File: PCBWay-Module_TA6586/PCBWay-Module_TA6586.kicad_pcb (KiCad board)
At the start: 2 copper layers, 16.3 x 20.8 mm, 4 parts, among them J1 Conn_01x07_Pin, J2 Conn_01x07_Pin

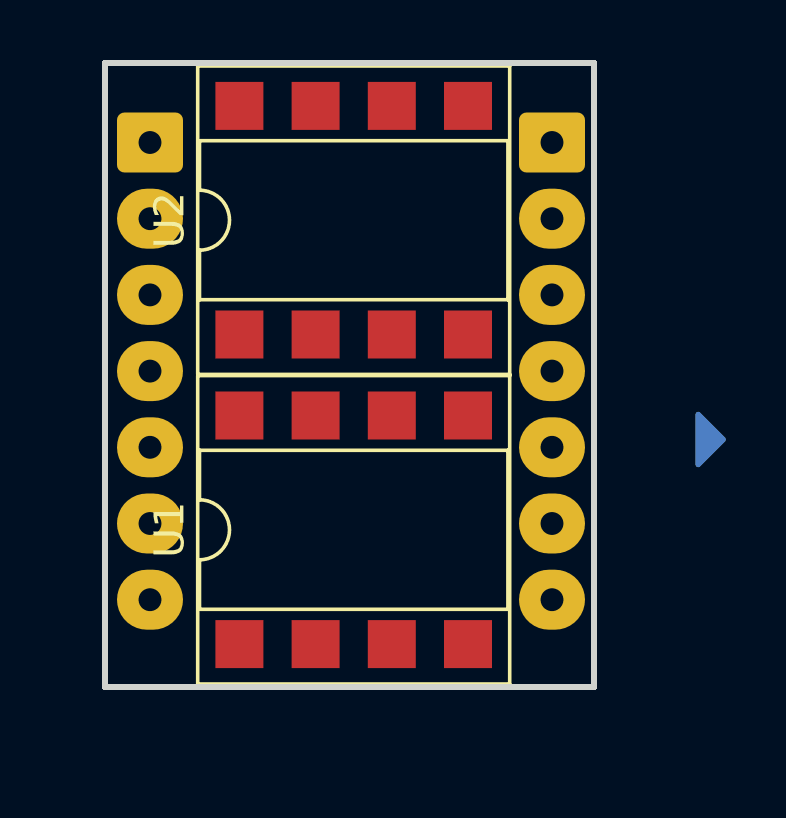
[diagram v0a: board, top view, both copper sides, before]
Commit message: the whole thing
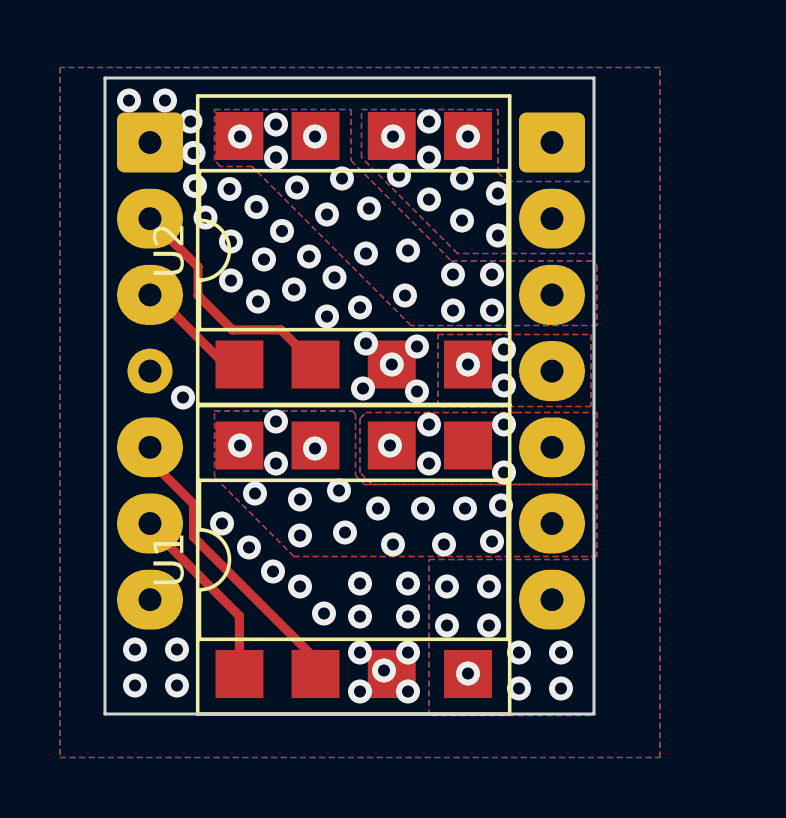
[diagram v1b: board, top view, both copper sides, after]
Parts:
- moved U1 1.00 mm to (146.8, 83.4)
- moved U2 1.00 mm to (146.8, 73.1)
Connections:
- J1 pad 4: unconnected-(J1-Pin_4-Pad4) -> (no net)
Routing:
- net /IN_A2: track 0.00 -> 9.85 mm
- net /IN_B2: track 0.00 -> 8.10 mm
- net /IN_A1: track 0.00 -> 6.25 mm
- net /IN_B1: track 0.00 -> 3.94 mm
- net GND: vias 0 -> 42
- net /VM: vias 0 -> 12
- net /OUT_B2: vias 0 -> 15
- net /OUT_B1: vias 0 -> 10
- net /OUT_A2: vias 0 -> 16
- net /OUT_A1: vias 0 -> 5
- added copper zone on B.Cu, net /OUT_A1
- added copper zone on F.Cu, net /OUT_A1
- added copper zone on B.Cu, net /OUT_A2
- added copper zone on F.Cu, net /OUT_A2
- added copper zone on B.Cu, net /OUT_B1
- added copper zone on F.Cu, net /OUT_B1
- added copper zone on B.Cu, net /OUT_B2
- added copper zone on F.Cu, net /OUT_B2
- added copper zone on B.Cu, net /VM
- added copper zone on F.Cu, net /VM
- added copper zone on B.Cu, net GND
- added copper zone on F.Cu, net GND
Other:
- board size 16.3 x 20.8 mm -> 16.3 x 21.2 mm
